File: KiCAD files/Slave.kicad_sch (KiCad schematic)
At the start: 11 parts, among them U5 NUCLEO64-F446RE

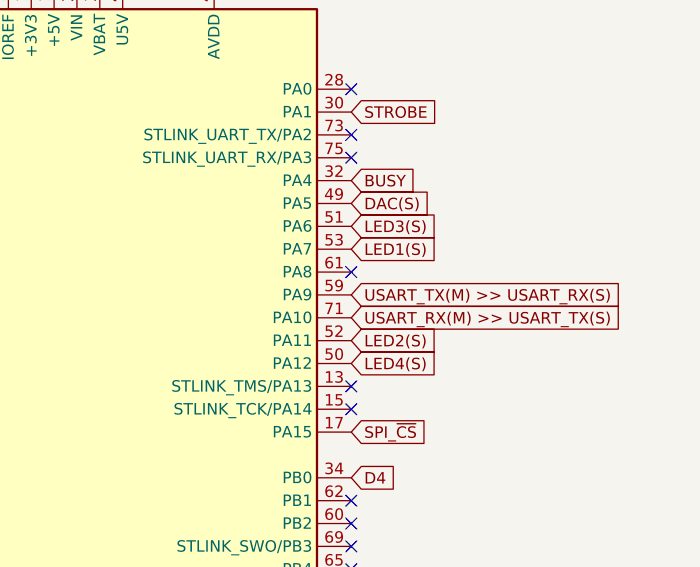
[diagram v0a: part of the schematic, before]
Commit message: update
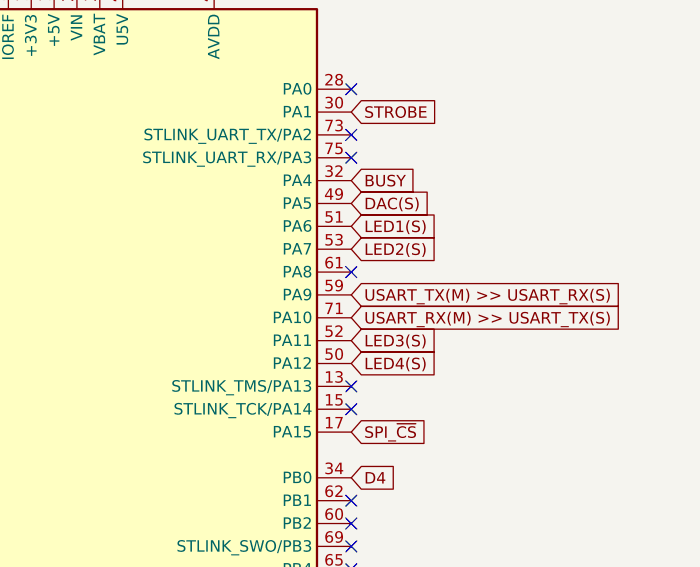
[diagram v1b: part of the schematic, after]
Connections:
- net LED1(S): now also U5.51 (PA6); no longer U5.53 (PA7)
- net LED2(S): now also U5.53 (PA7); no longer U5.52 (PA11)
- net LED3(S): now also U5.52 (PA11); no longer U5.51 (PA6)
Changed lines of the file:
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@@
     )
   )
-  (global_label "LED3(S)" (shape input) (at 172.72 71.12 0) (fields_autoplaced)
+  (global_label "LED3(S)" (shape input) (at 172.72 83.82 0) (fields_autoplaced)
     (effects (font (size 1.27 1.27)) (justify left))
-    (property "Intersheetrefs" "${INTERSHEET_REFS}" (at 183.2647 71.12 0)
+    (property "Intersheetrefs" "${INTERSHEET_REFS}" (at 183.2647 83.82 0)
       (effects (font (size 1.27 1.27)) (justify left) hide)
     )
@@
     )
   )
-  (global_label "LED2(S)" (shape input) (at 172.72 83.82 0) (fields_autoplaced)
+  (global_label "LED2(S)" (shape input) (at 172.72 73.66 0) (fields_autoplaced)
     (effects (font (size 1.27 1.27)) (justify left))
-    (property "Intersheetrefs" "${INTERSHEET_REFS}" (at 183.2647 83.82 0)
+    (property "Intersheetrefs" "${INTERSHEET_REFS}" (at 183.2647 73.66 0)
       (effects (font (size 1.27 1.27)) (justify left) hide)
     )
@@
     )
   )
-  (global_label "LED1(S)" (shape input) (at 172.72 73.66 0) (fields_autoplaced)
+  (global_label "LED1(S)" (shape input) (at 172.72 71.12 0) (fields_autoplaced)
     (effects (font (size 1.27 1.27)) (justify left))
-    (property "Intersheetrefs" "${INTERSHEET_REFS}" (at 183.2647 73.66 0)
+    (property "Intersheetrefs" "${INTERSHEET_REFS}" (at 183.2647 71.12 0)
       (effects (font (size 1.27 1.27)) (justify left) hide)
     )

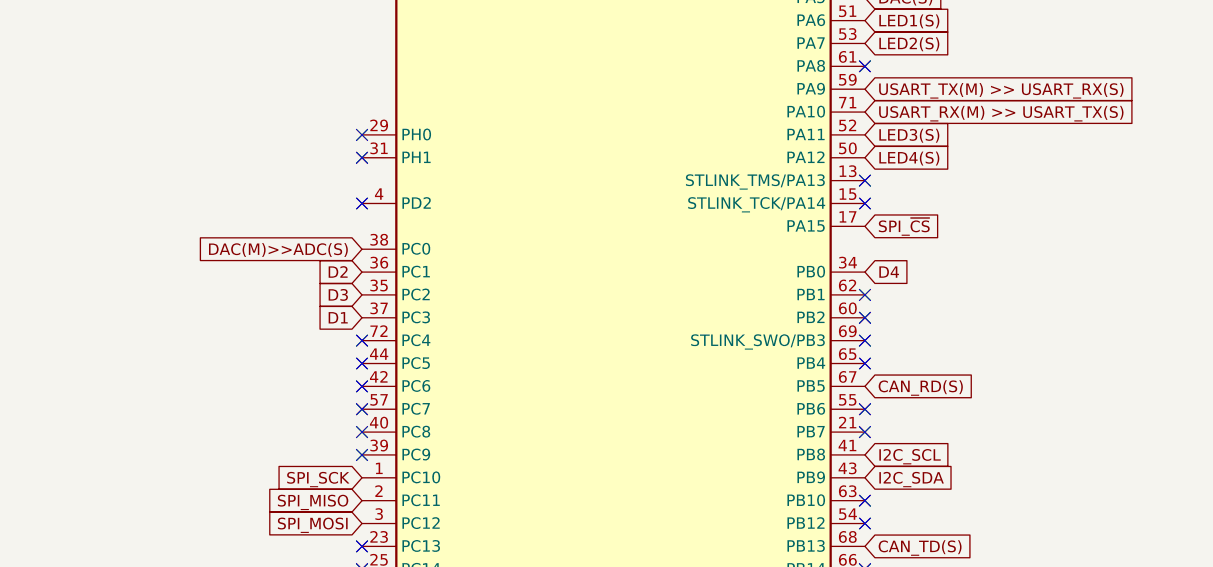
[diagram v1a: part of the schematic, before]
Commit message: update
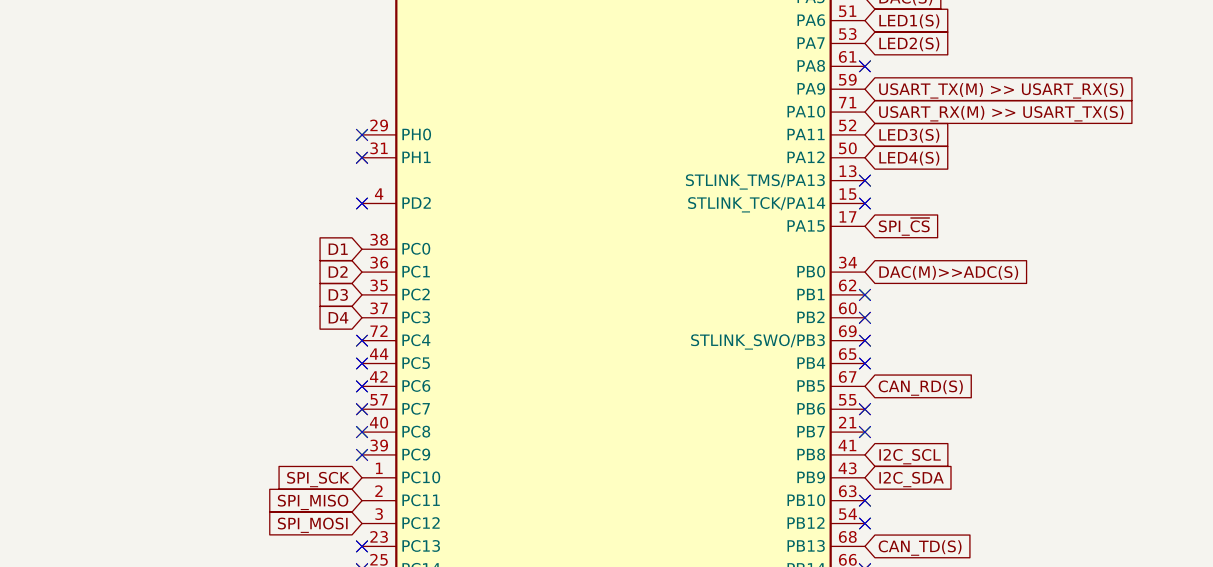
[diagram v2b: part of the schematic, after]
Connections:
- net D1: now also U5.38 (PC0); no longer U5.37 (PC3)
- net D4: now also U5.37 (PC3); no longer U5.34 (PB0)
- net DAC(M)>>ADC(S): now also U5.34 (PB0); no longer U5.38 (PC0)
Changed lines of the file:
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@@
   (no_connect (at 172.72 101.6))
   (no_connect (at 116.84 91.44))
-  (no_connect (at 116.84 106.68))
   (no_connect (at 172.72 106.68))
   (no_connect (at 172.72 91.44))
@@
   (no_connect (at 172.72 88.9))
   (no_connect (at 172.72 104.14))
+  (no_connect (at 116.84 106.68))
   (no_connect (at 147.32 43.18))
   (no_connect (at 172.72 76.2))
@@
     )
   )
-  (global_label "D1" (shape input) (at 116.84 104.14 180) (fields_autoplaced)
+  (global_label "D1" (shape input) (at 116.84 96.52 180) (fields_autoplaced)
+    (effects (font (size 1.27 1.27)) (justify right))
+    (property "Intersheetrefs" "${INTERSHEET_REFS}" (at 111.3753 96.52 0)
+      (effects (font (size 1.27 1.27)) (justify right) hide)
+    )
+  )
+  (global_label "DAC(M)>>ADC(S)" (shape input) (at 172.72 99.06 0) (fields_autoplaced)
+    (effects (font (size 1.27 1.27)) (justify left))
+    (property "Intersheetrefs" "${INTERSHEET_REFS}" (at 192.1549 99.06 0)
+      (effects (font (size 1.27 1.27)) (justify left) hide)
+    )
+  )
+  (global_label "LED4(S)" (shape input) (at 172.72 86.36 0) (fields_autoplaced)
+    (effects (font (size 1.27 1.27)) (justify left))
+    (property "Intersheetrefs" "${INTERSHEET_REFS}" (at 183.2647 86.36 0)
+      (effects (font (size 1.27 1.27)) (justify left) hide)
+    )
+  )
+  (global_label "CAN_RD(S)" (shape input) (at 172.72 111.76 0) (fields_autoplaced)
+    (effects (font (size 1.27 1.27)) (justify left))
+    (property "Intersheetrefs" "${INTERSHEET_REFS}" (at 185.8048 111.76 0)
+      (effects (font (size 1.27 1.27)) (justify left) hide)
+    )
+  )
+  (global_label "LED3(S)" (shape input) (at 172.72 83.82 0) (fields_autoplaced)
+    (effects (font (size 1.27 1.27)) (justify left))
+    (property "Intersheetrefs" "${INTERSHEET_REFS}" (at 183.2647 83.82 0)
+      (effects (font (size 1.27 1.27)) (justify left) hide)
+    )
+  )
+  (global_label "BUSY" (shape input) (at 172.72 66.04 0) (fields_autoplaced)
+    (effects (font (size 1.27 1.27)) (justify left))
+    (property "Intersheetrefs" "${INTERSHEET_REFS}" (at 180.6038 66.04 0)
+      (effects (font (size 1.27 1.27)) (justify left) hide)
+    )
+  )
+  (global_label "STROBE" (shape input) (at 172.72 58.42 0) (fields_autoplaced)
+    (effects (font (size 1.27 1.27)) (justify left))
+    (property "Intersheetrefs" "${INTERSHEET_REFS}" (at 182.9018 58.42 0)
+      (effects (font (size 1.27 1.27)) (justify left) hide)
+    )
+  )
+  (global_label "LED2(S)" (shape input) (at 172.72 73.66 0) (fields_autoplaced)
+    (effects (font (size 1.27 1.27)) (justify left))
+    (property "Intersheetrefs" "${INTERSHEET_REFS}" (at 183.2647 73.66 0)
+      (effects (font (size 1.27 1.27)) (justify left) hide)
+    )
+  )
+  (global_label "USART_RX(M) >> USART_TX(S)" (shape input) (at 172.72 81.28 0) (fields_autoplaced)
+    (effects (font (size 1.27 1.27)) (justify left))
+    (property "Intersheetrefs" "${INTERSHEET_REFS}" (at 205.1571 81.28 0)
+      (effects (font (size 1.27 1.27)) (justify left) hide)
+    )
+  )
+  (global_label "LED3(S)" (shape input) (at 45.085 70.485 90) (fields_autoplaced)
+    (effects (font (size 1.27 1.27)) (justify left))
+    (property "Intersheetrefs" "${INTERSHEET_REFS}" (at 45.085 59.9403 90)
+      (effects (font (size 1.27 1.27)) (justify left) hide)
+    )
+  )
+  (global_label "DAC(S)" (shape input) (at 172.72 68.58 0) (fields_autoplaced)
+    (effects (font (size 1.27 1.27)) (justify left))
+    (property "Intersheetrefs" "${INTERSHEET_REFS}" (at 182.2367 68.58 0)
+      (effects (font (size 1.27 1.27)) (justify left) hide)
+    )
+  )
+  (global_label "D4" (shape input) (at 116.84 104.14 180) (fields_autoplaced)
     (effects (font (size 1.27 1.27)) (justify right))
     (property "Intersheetrefs" "${INTERSHEET_REFS}" (at 111.3753 104.14 0)
@@
     )
   )
-  (global_label "DAC(M)>>ADC(S)" (shape input) (at 116.84 96.52 180) (fields_autoplaced)
-    (effects (font (size 1.27 1.27)) (justify right))
-    (property "Intersheetrefs" "${INTERSHEET_REFS}" (at 97.4051 96.52 0)
-      (effects (font (size 1.27 1.27)) (justify right) hide)
-    )
-  )
-  (global_label "LED4(S)" (shape input) (at 172.72 86.36 0) (fields_autoplaced)
-    (effects (font (size 1.27 1.27)) (justify left))
-    (property "Intersheetrefs" "${INTERSHEET_REFS}" (at 183.2647 86.36 0)
-      (effects (font (size 1.27 1.27)) (justify left) hide)
-    )
-  )
-  (global_label "CAN_RD(S)" (shape input) (at 172.72 111.76 0) (fields_autoplaced)
-    (effects (font (size 1.27 1.27)) (justify left))
-    (property "Intersheetrefs" "${INTERSHEET_REFS}" (at 185.8048 111.76 0)
-      (effects (font (size 1.27 1.27)) (justify left) hide)
-    )
-  )
-  (global_label "LED3(S)" (shape input) (at 172.72 83.82 0) (fields_autoplaced)
-    (effects (font (size 1.27 1.27)) (justify left))
-    (property "Intersheetrefs" "${INTERSHEET_REFS}" (at 183.2647 83.82 0)
-      (effects (font (size 1.27 1.27)) (justify left) hide)
-    )
-  )
-  (global_label "BUSY" (shape input) (at 172.72 66.04 0) (fields_autoplaced)
-    (effects (font (size 1.27 1.27)) (justify left))
-    (property "Intersheetrefs" "${INTERSHEET_REFS}" (at 180.6038 66.04 0)
-      (effects (font (size 1.27 1.27)) (justify left) hide)
-    )
-  )
-  (global_label "STROBE" (shape input) (at 172.72 58.42 0) (fields_autoplaced)
-    (effects (font (size 1.27 1.27)) (justify left))
-    (property "Intersheetrefs" "${INTERSHEET_REFS}" (at 182.9018 58.42 0)
-      (effects (font (size 1.27 1.27)) (justify left) hide)
-    )
-  )
-  (global_label "LED2(S)" (shape input) (at 172.72 73.66 0) (fields_autoplaced)
-    (effects (font (size 1.27 1.27)) (justify left))
-    (property "Intersheetrefs" "${INTERSHEET_REFS}" (at 183.2647 73.66 0)
-      (effects (font (size 1.27 1.27)) (justify left) hide)
-    )
-  )
-  (global_label "USART_RX(M) >> USART_TX(S)" (shape input) (at 172.72 81.28 0) (fields_autoplaced)
-    (effects (font (size 1.27 1.27)) (justify left))
-    (property "Intersheetrefs" "${INTERSHEET_REFS}" (at 205.1571 81.28 0)
-      (effects (font (size 1.27 1.27)) (justify left) hide)
-    )
-  )
-  (global_label "LED3(S)" (shape input) (at 45.085 70.485 90) (fields_autoplaced)
-    (effects (font (size 1.27 1.27)) (justify left))
-    (property "Intersheetrefs" "${INTERSHEET_REFS}" (at 45.085 59.9403 90)
-      (effects (font (size 1.27 1.27)) (justify left) hide)
-    )
-  )
-  (global_label "DAC(S)" (shape input) (at 172.72 68.58 0) (fields_autoplaced)
-    (effects (font (size 1.27 1.27)) (justify left))
-    (property "Intersheetrefs" "${INTERSHEET_REFS}" (at 182.2367 68.58 0)
-      (effects (font (size 1.27 1.27)) (justify left) hide)
-    )
-  )
-  (global_label "D4" (shape input) (at 172.72 99.06 0) (fields_autoplaced)
-    (effects (font (size 1.27 1.27)) (justify left))
-    (property "Intersheetrefs" "${INTERSHEET_REFS}" (at 178.1847 99.06 0)
-      (effects (font (size 1.27 1.27)) (justify left) hide)
-    )
-  )

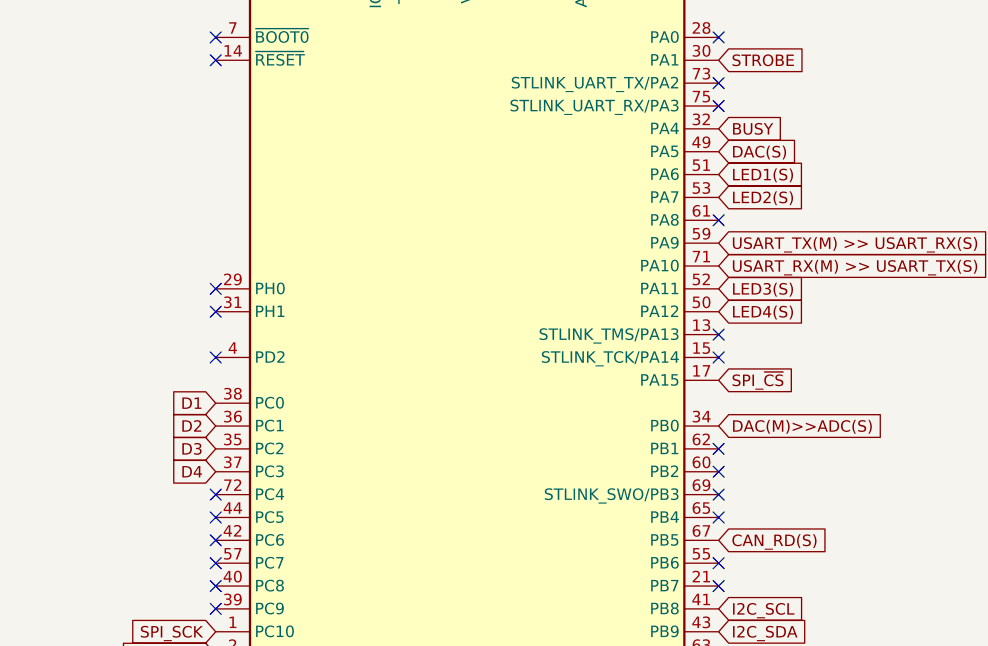
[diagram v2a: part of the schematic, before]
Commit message: update
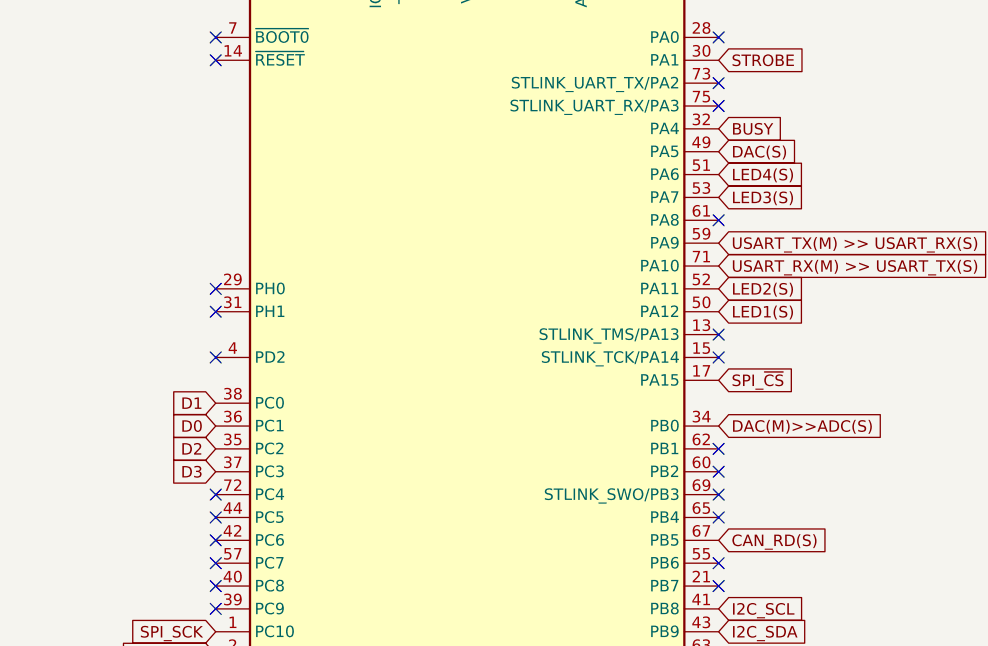
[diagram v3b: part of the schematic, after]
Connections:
- net D4 is gone; now on net D3: U5.37 (PC3)
- net D2: now also U5.35 (PC2); no longer U5.36 (PC1)
- net D3: no longer U5.35 (PC2)
- net LED1(S): now also U5.50 (PA12); no longer U5.51 (PA6)
- net LED2(S): now also U5.52 (PA11); no longer U5.53 (PA7)
- net LED3(S): now also U5.53 (PA7); no longer U5.52 (PA11)
- net LED4(S): now also U5.51 (PA6); no longer U5.50 (PA12)
- new net D0: U5.36 (PC1)
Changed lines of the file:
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@@
     )
   )
-  (global_label "D2" (shape input) (at 116.84 99.06 180) (fields_autoplaced)
+  (global_label "D1" (shape input) (at 116.84 96.52 180) (fields_autoplaced)
     (effects (font (size 1.27 1.27)) (justify right))
-    (property "Intersheetrefs" "${INTERSHEET_REFS}" (at 111.3753 99.06 0)
+    (property "Intersheetrefs" "${INTERSHEET_REFS}" (at 111.3753 96.52 0)
       (effects (font (size 1.27 1.27)) (justify right) hide)
     )
@@
     )
   )
-  (global_label "D1" (shape input) (at 116.84 96.52 180) (fields_autoplaced)
+  (global_label "D0" (shape input) (at 116.84 99.06 180) (fields_autoplaced)
     (effects (font (size 1.27 1.27)) (justify right))
-    (property "Intersheetrefs" "${INTERSHEET_REFS}" (at 111.3753 96.52 0)
+    (property "Intersheetrefs" "${INTERSHEET_REFS}" (at 111.3753 99.06 0)
       (effects (font (size 1.27 1.27)) (justify right) hide)
     )
@@
     )
   )
-  (global_label "LED4(S)" (shape input) (at 172.72 86.36 0) (fields_autoplaced)
+  (global_label "LED4(S)" (shape input) (at 172.72 71.12 0) (fields_autoplaced)
     (effects (font (size 1.27 1.27)) (justify left))
-    (property "Intersheetrefs" "${INTERSHEET_REFS}" (at 183.2647 86.36 0)
+    (property "Intersheetrefs" "${INTERSHEET_REFS}" (at 183.2647 71.12 0)
       (effects (font (size 1.27 1.27)) (justify left) hide)
     )
@@
     )
   )
-  (global_label "LED3(S)" (shape input) (at 172.72 83.82 0) (fields_autoplaced)
+  (global_label "LED3(S)" (shape input) (at 172.72 73.66 0) (fields_autoplaced)
     (effects (font (size 1.27 1.27)) (justify left))
-    (property "Intersheetrefs" "${INTERSHEET_REFS}" (at 183.2647 83.82 0)
+    (property "Intersheetrefs" "${INTERSHEET_REFS}" (at 183.2647 73.66 0)
       (effects (font (size 1.27 1.27)) (justify left) hide)
     )
@@
     )
   )
-  (global_label "LED2(S)" (shape input) (at 172.72 73.66 0) (fields_autoplaced)
+  (global_label "LED2(S)" (shape input) (at 172.72 83.82 0) (fields_autoplaced)
     (effects (font (size 1.27 1.27)) (justify left))
-    (property "Intersheetrefs" "${INTERSHEET_REFS}" (at 183.2647 73.66 0)
+    (property "Intersheetrefs" "${INTERSHEET_REFS}" (at 183.2647 83.82 0)
       (effects (font (size 1.27 1.27)) (justify left) hide)
     )
@@
     )
   )
-  (global_label "D4" (shape input) (at 116.84 104.14 180) (fields_autoplaced)
+  (global_label "D3" (shape input) (at 116.84 104.14 180) (fields_autoplaced)
     (effects (font (size 1.27 1.27)) (justify right))
     (property "Intersheetrefs" "${INTERSHEET_REFS}" (at 111.3753 104.14 0)
@@
     )
   )
-  (global_label "D3" (shape input) (at 116.84 101.6 180) (fields_autoplaced)
+  (global_label "D2" (shape input) (at 116.84 101.6 180) (fields_autoplaced)
     (effects (font (size 1.27 1.27)) (justify right))
     (property "Intersheetrefs" "${INTERSHEET_REFS}" (at 111.3753 101.6 0)
@@
     )
   )
-  (global_label "LED1(S)" (shape input) (at 172.72 71.12 0) (fields_autoplaced)
+  (global_label "LED1(S)" (shape input) (at 172.72 86.36 0) (fields_autoplaced)
     (effects (font (size 1.27 1.27)) (justify left))
-    (property "Intersheetrefs" "${INTERSHEET_REFS}" (at 183.2647 71.12 0)
+    (property "Intersheetrefs" "${INTERSHEET_REFS}" (at 183.2647 86.36 0)
       (effects (font (size 1.27 1.27)) (justify left) hide)
     )
